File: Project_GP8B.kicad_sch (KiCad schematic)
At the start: 15 parts, among them U1 74AHC05, U2 74AHC05, U5 74AHC05

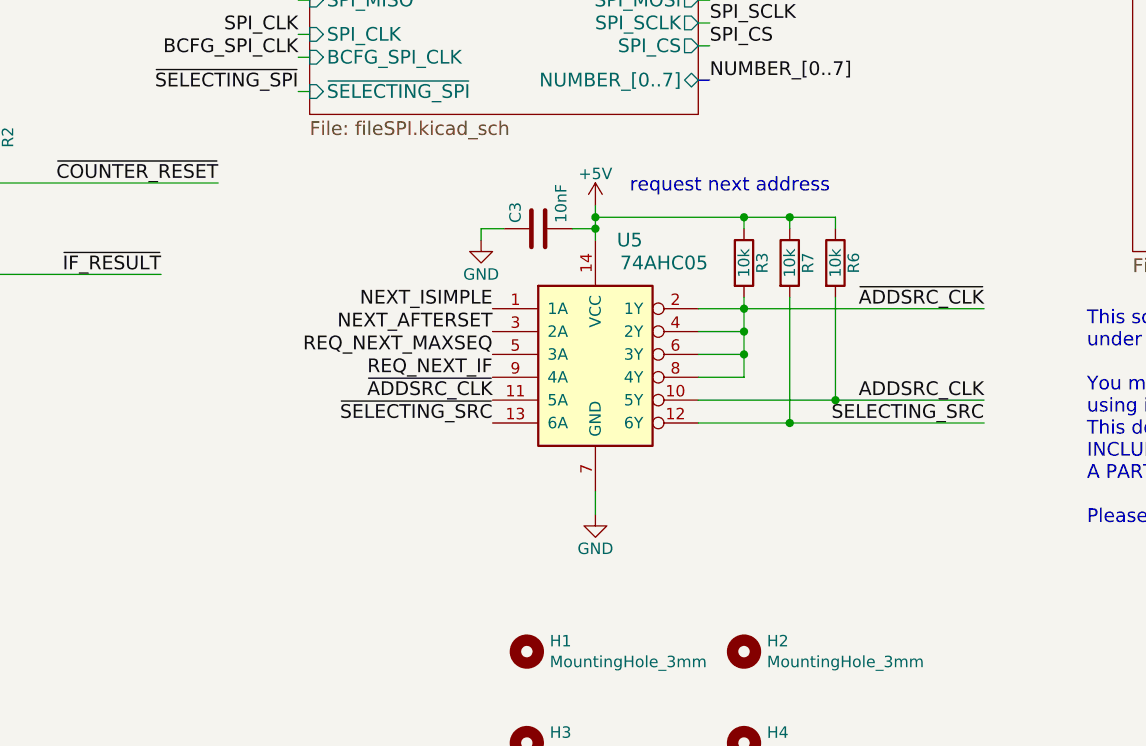
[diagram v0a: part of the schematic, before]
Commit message: bit of cleaning after last commit
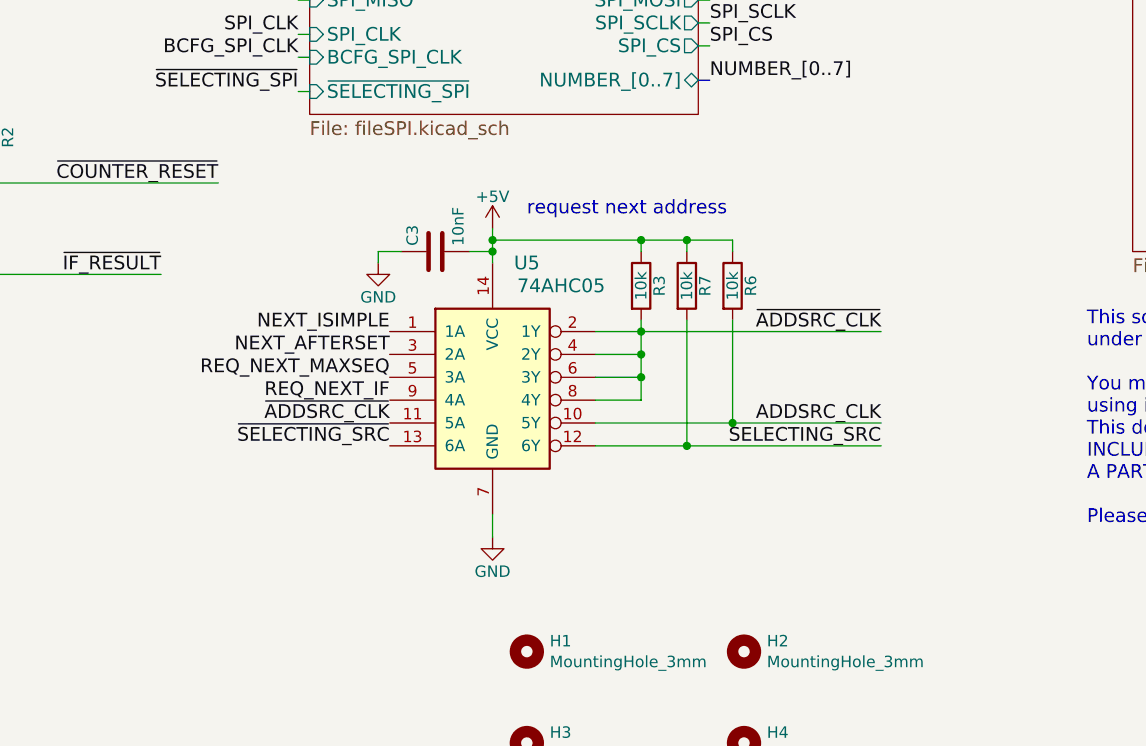
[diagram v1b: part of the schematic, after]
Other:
- moved on the sheet: C3, R3, R6, R7, U5
